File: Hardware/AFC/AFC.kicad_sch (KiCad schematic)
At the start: 59 parts, among them J1 Barrel_Jack_Switch, J2 Conn_Coaxial, J3 Conn_Coaxial, J4 Conn_Coaxial, J5 Conn_Coaxial, U1 AD633JRZ, U2 AD633JRZ, U3 AD630ARZ, U4 AD8429, U5 AD8429, U6 LM358, U7 LM358

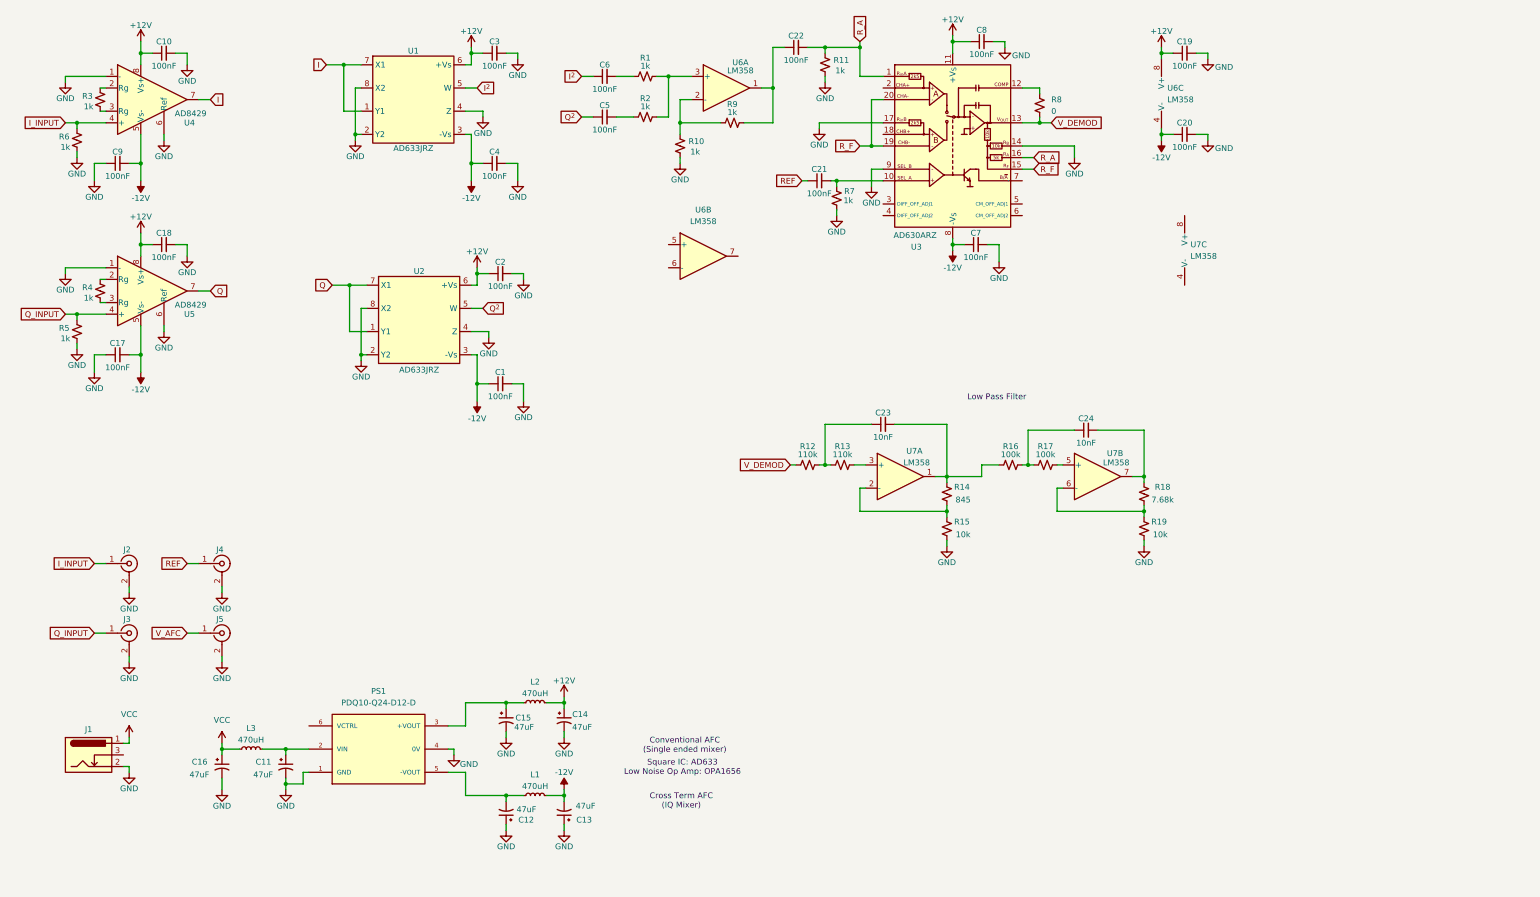
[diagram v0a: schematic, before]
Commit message: Updates to AFC schematic
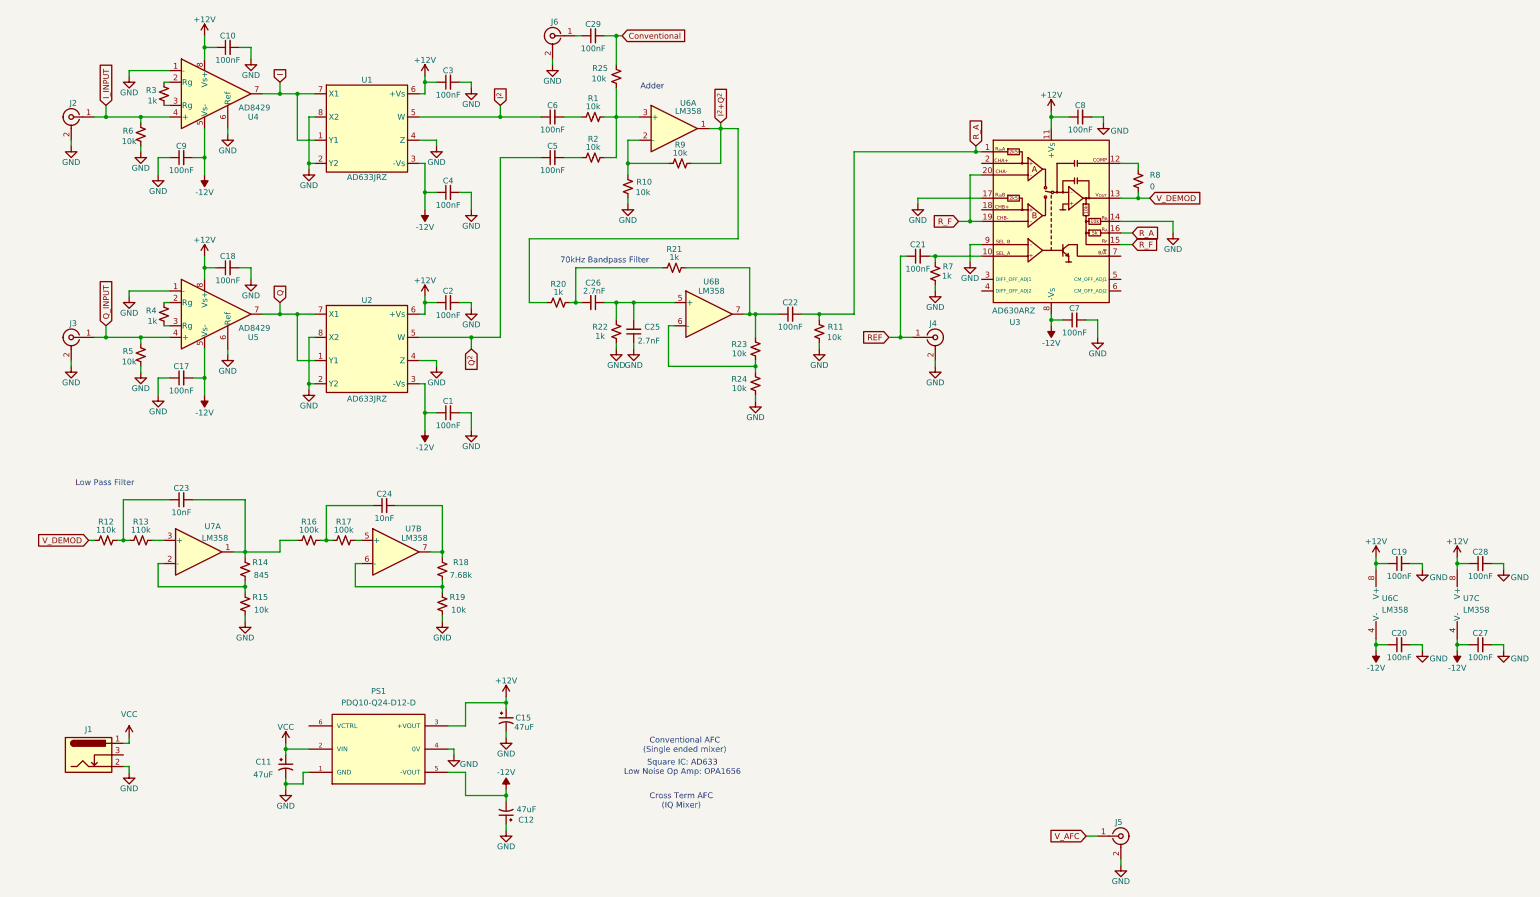
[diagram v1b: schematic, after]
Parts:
- removed C13, C14, C16: 47uF, symbol Device:C_Polarized_Small_US
- removed L1, L2, L3: 470uH, symbol Device:L_Small
- added C25, C26: 2.7nF, symbol Device:C_Small
- added C27, C28, C29: 100nF, symbol Device:C_Small
- added J6: Conn_Coaxial, symbol Connector:Conn_Coaxial
- added R20, R21, R22: 1k, symbol Device:R_Small_US
- added R23, R24, R25: 10k, symbol Device:R_Small_US
- R1, R10, R11, R2, R5, R6, R9: value 1k -> 10k
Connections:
- net +12V: now also C15.1, PS1.3 (+VOUT), U7.8 (V+), C28.1
- net -12V: now also C12.2, PS1.5 (-VOUT), U7.4 (V-), C27.1
- net GND: now also C25.1, C27.2, C28.2, J6.2 (Ext), R22.1, R24.1
- net VCC: now also C11.1, PS1.2 (VIN)
- net at R1.2, R2.2, U6.3 (+): now also R25.2
- net I^{2}+Q^{2}: now reaches R9.2, U6.1
- net I^{2}+Q^{2}: now also R20.1; no longer C22.1
- net at U6.5 (+): now also C25.2, C26.1, R22.2
- net at U6.6 (-): now also R23.1, R24.2
- net at U6.7: now also C22.1, R21.2, R23.2
- new net: C29.1, J6.1 (In)
- new net: C26.2, R20.2, R21.1
- new net Conventional: C29.2, R25.1
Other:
- note added: "70kHz Bandpass Filter"
- note added: "Adder"
- moved on the sheet: C1, C10, C17, C18, C19, C2, C20, C21, C22, C23, C24, C3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
